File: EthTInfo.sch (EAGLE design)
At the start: 11 parts, among them J1 1X2-3.5MM-3.5MM, Q1 BSS138

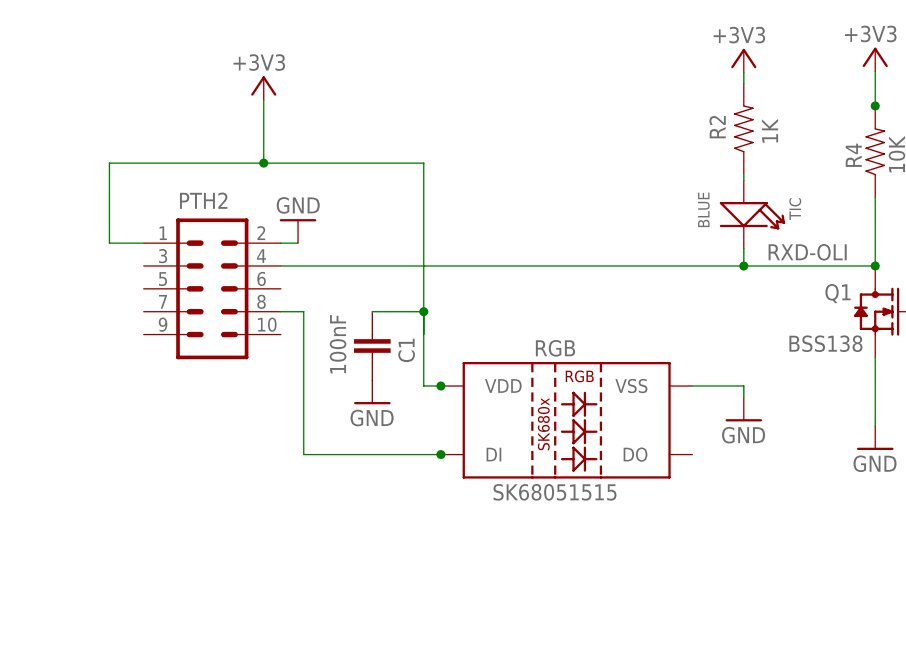
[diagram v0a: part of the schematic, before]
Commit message: Bump to V1.1
Bump to V1.1
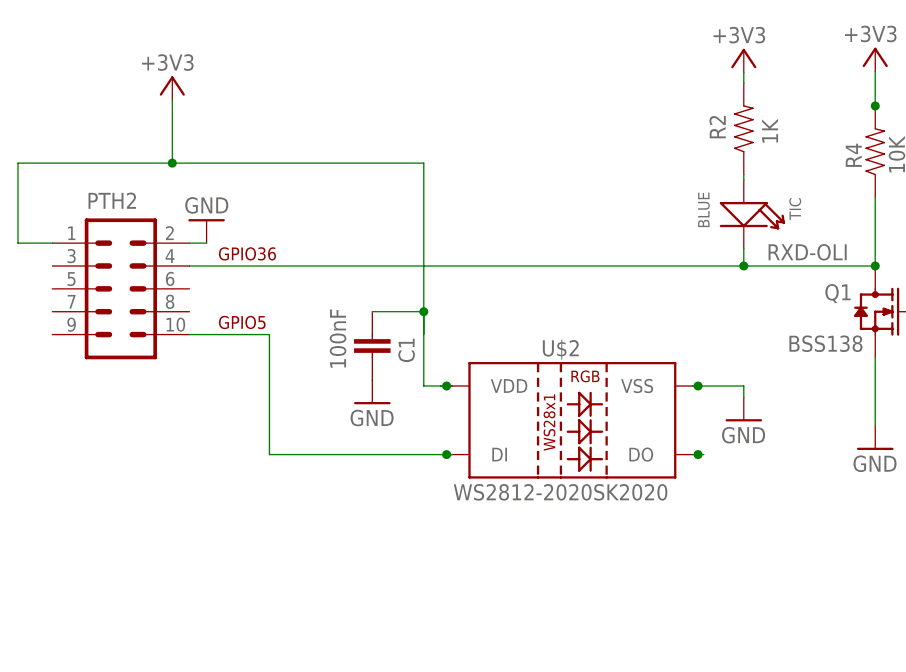
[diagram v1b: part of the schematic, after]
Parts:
- removed RGB: SK68051515, _c2h:SK68051515
- added U$2: WS2812-2020SK2020, _c2h:WS2812-2020SK2020
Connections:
- new net N$5: U$2.DO
- net 3V3: now also U$2.VDD; no longer RGB.VDD
- net GND: now also U$2.VSS; no longer RGB.VSS
- net N$6: now also PTH2.10, U$2.DI; no longer PTH2.8, RGB.DI
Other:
- note added: "GPIO36"
- note added: "GPIO5"
- moved on the sheet: PTH2
